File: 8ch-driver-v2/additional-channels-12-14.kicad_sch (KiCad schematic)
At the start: 42 parts, among them Q12 2N7002E, Q13 2N7002E, Q14 2N7002E, U12 DRV104PWP, U13 DRV104PWP, U14 DRV104PWP

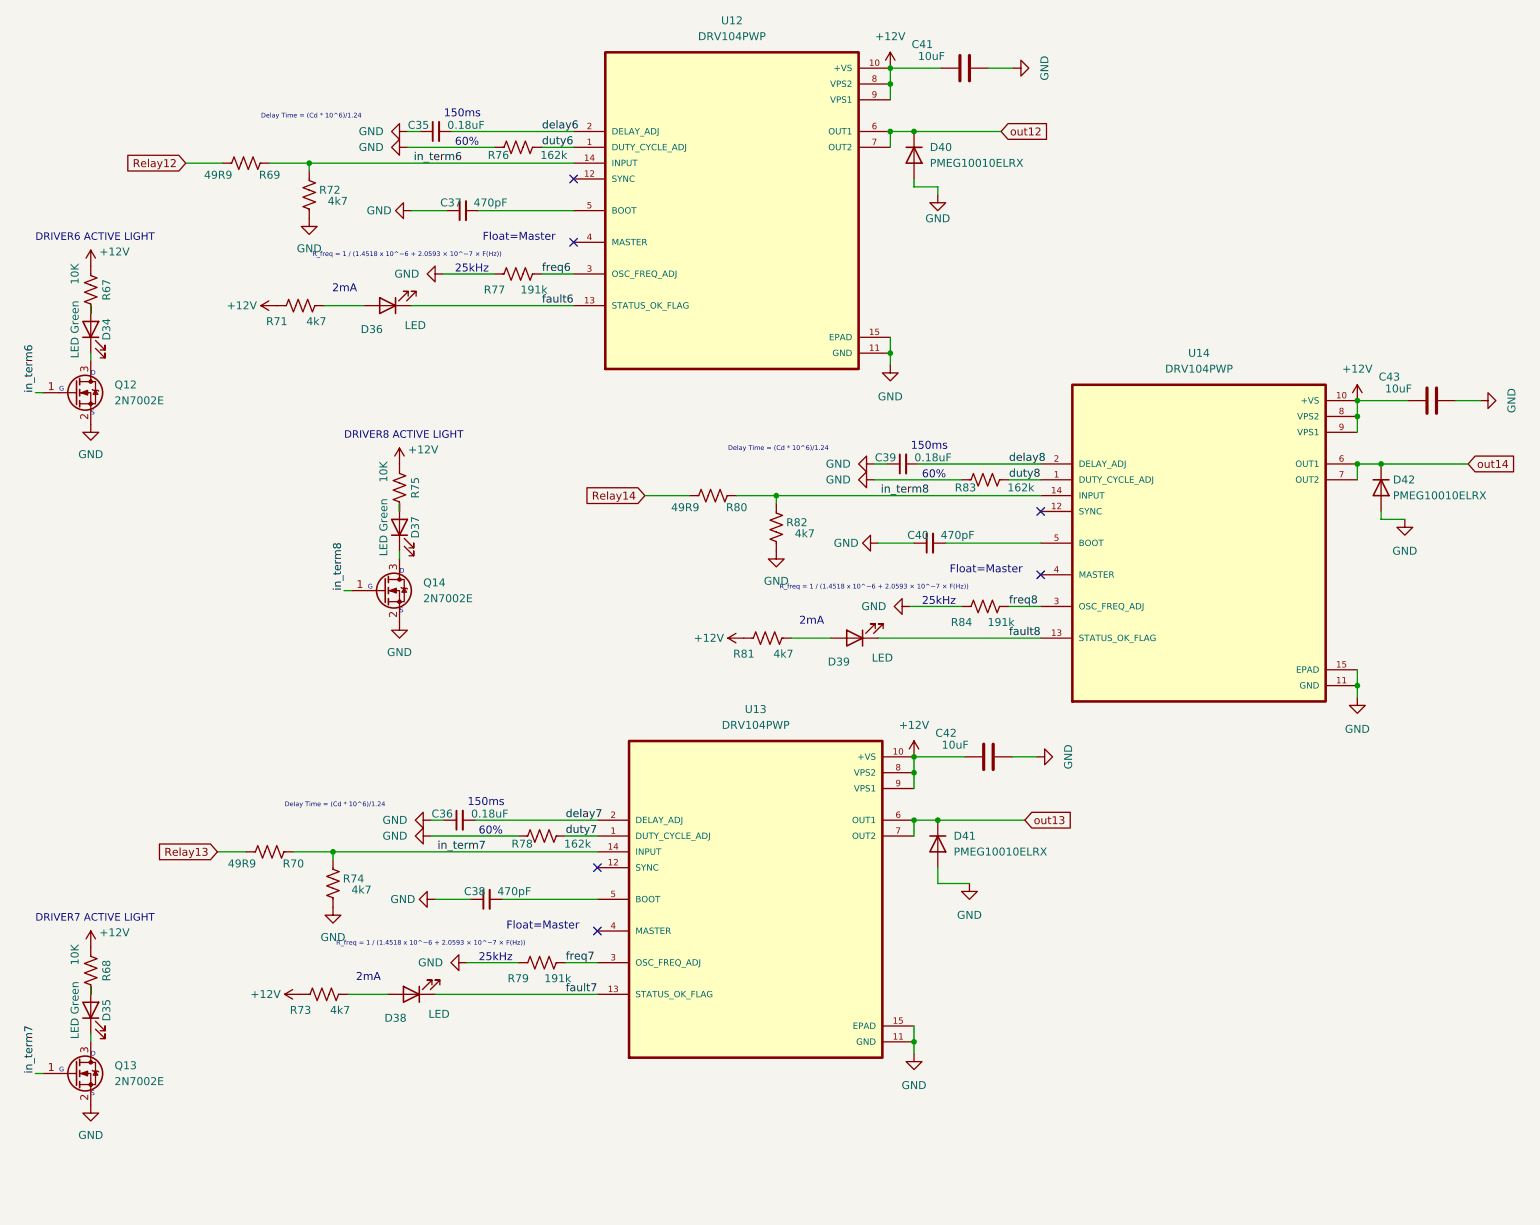
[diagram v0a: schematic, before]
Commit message: mucho mas progresso
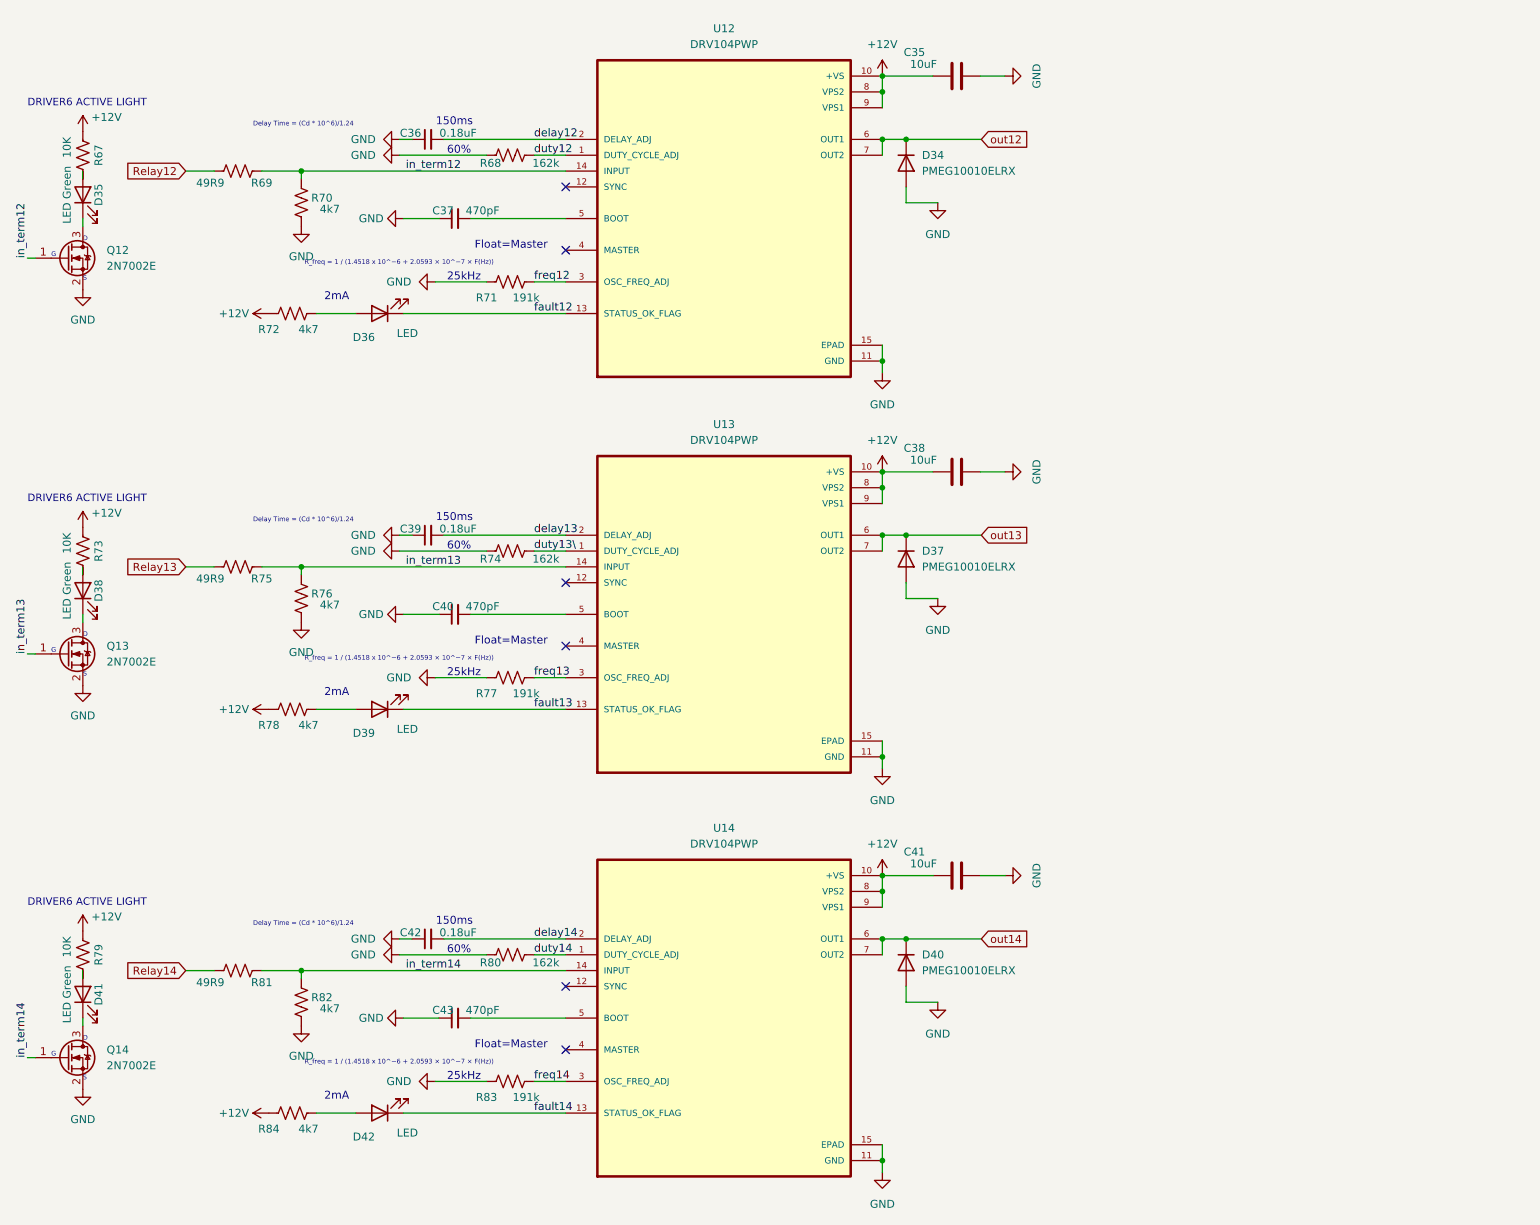
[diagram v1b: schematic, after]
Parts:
- removed C35: 0.18uF, Capacitor_SMD:C_1206_3216Metric, symbol Device:C_Small
- removed C38: 470pF, Capacitor_SMD:C_1206_3216Metric, symbol Device:C_Small
- removed C42, C43: 10uF, Capacitor_SMD:C_1210_3225Metric, symbol Device:C
- removed D34, D37: LED Green, LED_SMD:LED_0805_2012Metric, symbol Device:LED
- removed D41, D42: PMEG10010ELRX, Diode_SMD:Nexperia_CFP3_SOD-123W, symbol Device:D
- added C35, C38: 10uF, Capacitor_SMD:C_1210_3225Metric, symbol Device:C
- added C42: 0.18uF, Capacitor_SMD:C_1206_3216Metric, symbol Device:C_Small
- added C43: 470pF, Capacitor_SMD:C_1206_3216Metric, symbol Device:C_Small
- added D34, D37: PMEG10010ELRX, Diode_SMD:Nexperia_CFP3_SOD-123W, symbol Device:D
- added D41: LED Green, LED_SMD:LED_0805_2012Metric, symbol Device:LED
- added D42: LED, LED_SMD:LED_0805_2012Metric, symbol Device:LED
- D38: value LED -> LED Green
- R68: value 10K -> 162k
- R70: value 49R9 -> 4k7; PartNum RC0805FR-0749R9L -> RC0805JR-074K7L
- R71: value 4k7 -> 191k; PartNum RC0805JR-074K7L -> RC0805FR-07191KL
- R73: value 4k7 -> 10K; PartNum RC0805JR-074K7L -> RC0805FR-07162KL
- R74: value 4k7 -> 162k; PartNum RC0805JR-074K7L -> RC0805FR-07162KL
- R75: value 10K -> 49R9; PartNum RC0805FR-07162KL -> RC0805FR-0749R9L
- R76, R78: value 162k -> 4k7; PartNum RC0805FR-07162KL -> RC0805JR-074K7L
- R79: value 191k -> 10K; PartNum RC0805FR-07191KL -> RC0805FR-07162KL
- R80: value 49R9 -> 162k; PartNum RC0805FR-0749R9L -> RC0805FR-07162KL
- R81: value 4k7 -> 49R9; PartNum RC0805JR-074K7L -> RC0805FR-0749R9L
- R83: value 162k -> 191k; PartNum RC0805FR-07162KL -> RC0805FR-07191KL
- R84: value 191k -> 4k7; PartNum RC0805FR-07191KL -> RC0805JR-074K7L
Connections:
- net +12V: now also R72.1, R78.1, R79.1, R84.1, C35.1, C38.1; no longer R68.1, R71.1, R75.1, R81.1
- net GND: now also R68.1, R70.1, R71.1, R80.1, C35.2, C38.2, C42.1, C43.1, D34.2 (A), D37.2 (A); no longer R72.1, R78.1, R79.1, R84.1
- net Relay13: now also R75.1; no longer R70.1
- net Relay14: now also R81.1; no longer R80.1
- net out12: now also D34.1 (K); no longer D40.1 (K)
- net out13: now also D37.1 (K)
- net out14: now also D40.1 (K)
- net at Q12.3 (D): now also D35.1 (K)
- net at D36.2 (A): now also R72.2; no longer R71.2
- net at R67.2: now also D35.2 (A)
- net at C40.2: now also U13.5 (BOOT); no longer U14.5 (BOOT)
- net in_term13: now reaches R75.2
- net in_term13: now also Q13.1 (G), R76.2, U13.14 (INPUT)
- net at Q14.3 (D): now also D41.1 (K)
- net at D39.2 (A): now also R78.2; no longer R81.2
- net at Q13.3 (D): now also D38.1 (K); no longer D35.1 (K)
- net duty12: now reaches R68.2
- net duty12: now also U12.1 (DUTY_CYCLE_ADJ); no longer D35.2 (A)
- net delay6 renamed delay12
- net delay12: now also C36.2
- net delay7 renamed delay13
- net delay13: now also C39.2; no longer C36.2
- net delay8 renamed delay14
- net delay14: now also C42.2; no longer C39.2
- removed net duty6: R76.2, U12.1 (DUTY_CYCLE_ADJ)
- net duty7 renamed duty13\
- net duty13\: now also R74.2; no longer R78.2
- net duty8 renamed duty14
- net duty14: now also R80.2; no longer R83.2
- net fault6 renamed fault12
- net fault7 renamed fault13
- net fault13: now also D39.1 (K); no longer D38.1 (K)
- net fault8 renamed fault14
- net fault14: now also D42.1 (K); no longer D39.1 (K)
- net freq6 renamed freq12
- net freq12: now also R71.2; no longer R77.2
- net freq7: no longer names the net of R79.2
- net freq7: now also D41.2 (A); no longer U13.3 (OSC_FREQ_ADJ)
- net freq8: no longer names the net of R84.2
- net freq8: now also D42.2 (A); no longer U14.3 (OSC_FREQ_ADJ)
- net in_term6 renamed in_term12
- net in_term12: now also R70.2; no longer R72.2
- removed net in_term7: Q13.1 (G), R70.2, R74.2, U13.14 (INPUT)
- net in_term8 renamed in_term14
- net in_term14: now also R81.2; no longer R80.2
- new net: C43.2, U14.5 (BOOT)
- new net freq13: R77.2, U13.3 (OSC_FREQ_ADJ)
- new net freq14: R83.2, U14.3 (OSC_FREQ_ADJ)
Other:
- note removed: "DRIVER7 ACTIVE LIGHT"
- note removed: "DRIVER8 ACTIVE LIGHT"
